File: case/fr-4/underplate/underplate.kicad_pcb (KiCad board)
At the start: 2 copper layers, 152.3 x 104.7 mm, 8 parts

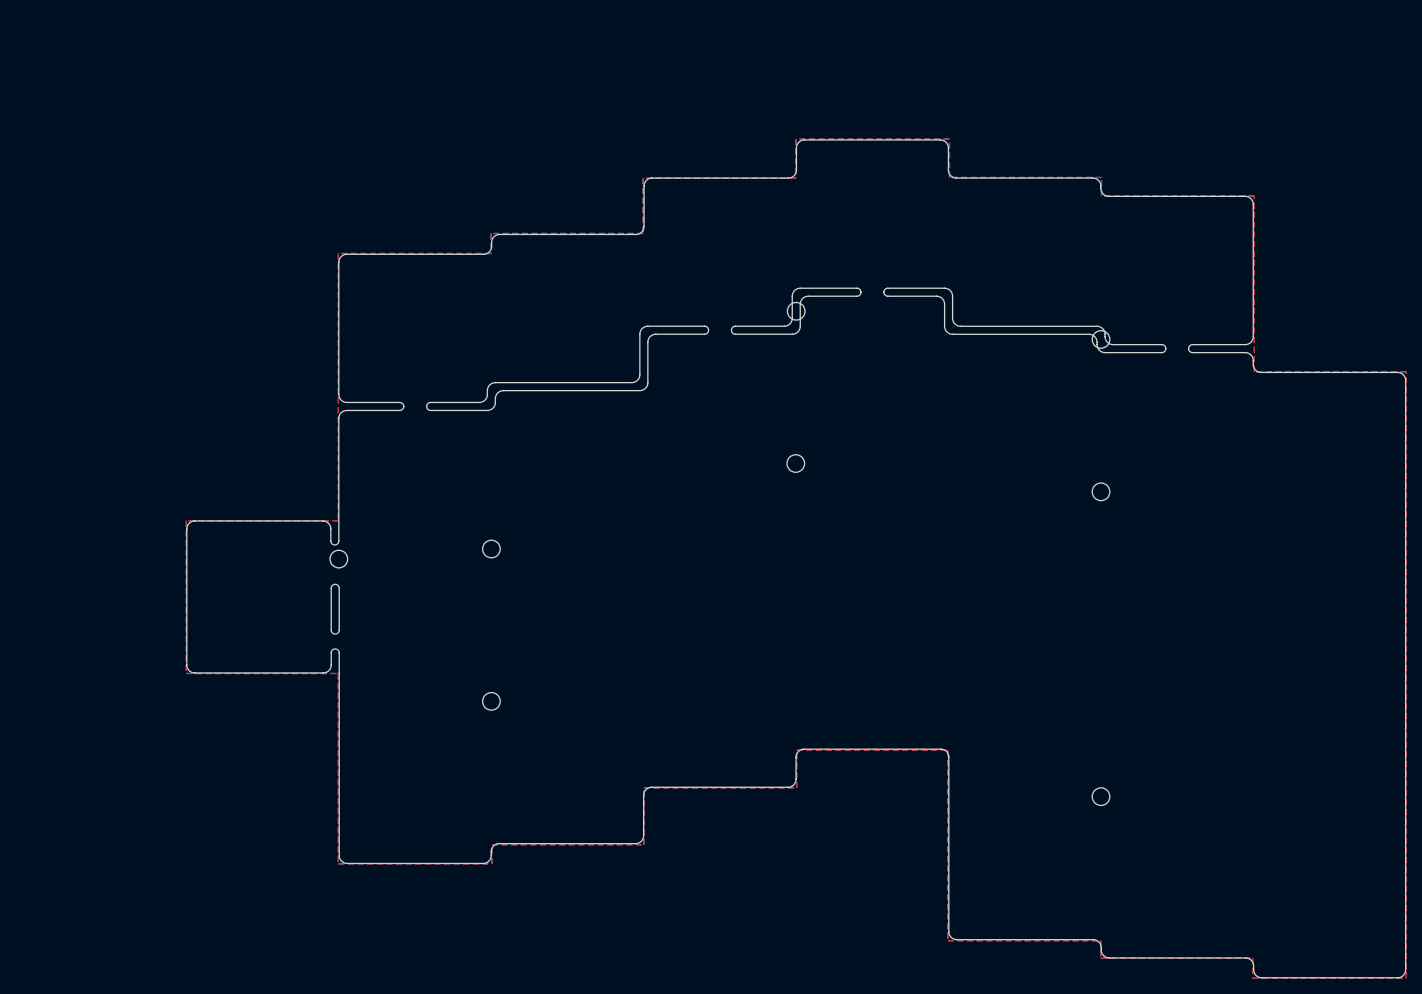
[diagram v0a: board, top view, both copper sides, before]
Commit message: Change screw holes
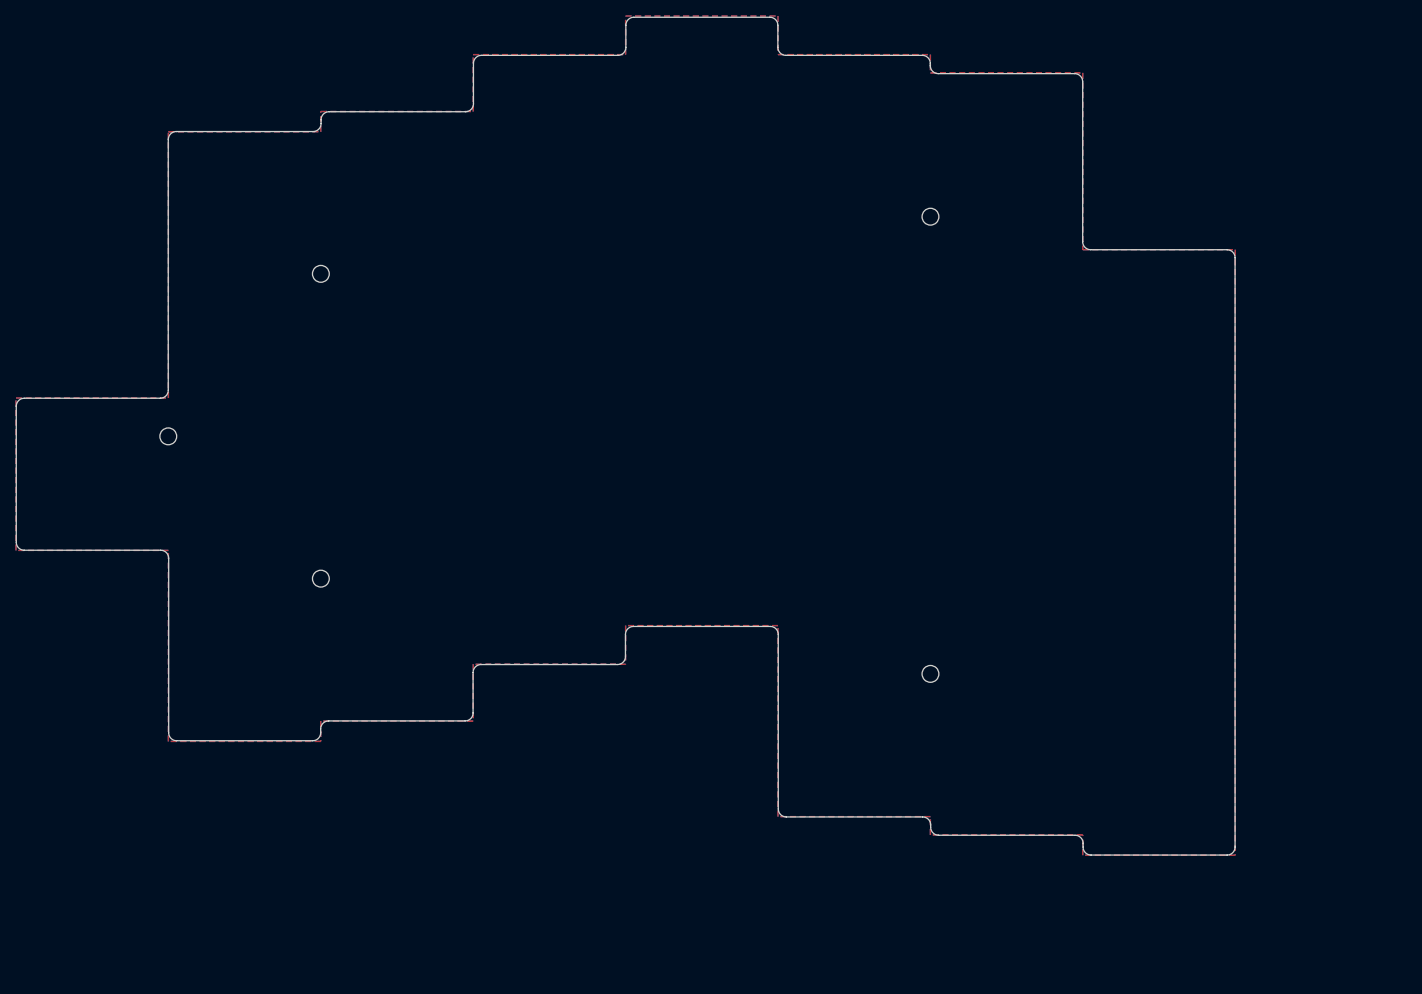
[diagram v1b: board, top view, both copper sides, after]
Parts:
- removed HM1, HM2, HM3, HM4, HM5, HM6, HM7, HM8: CaseHole, Used_Footprints:Hole_Mount_M4
- added REF**: MountingHole_2.1mm, MountingHole:MountingHole_2.1mm, F.Cu at (83.5, 95.2)
- added REF**: MountingHole_2.1mm, MountingHole:MountingHole_2.1mm, F.Cu at (178.8, 124.9)
- added REF**: MountingHole_2.1mm, MountingHole:MountingHole_2.1mm, F.Cu at (178.8, 67.8)
- added REF**: MountingHole_2.1mm, MountingHole:MountingHole_2.1mm, F.Cu at (102.6, 74.9)
- added REF**: MountingHole_2.1mm, MountingHole:MountingHole_2.1mm, F.Cu at (102.6, 113.0)
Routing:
- net (no net): vias 0 -> 1
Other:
- board size 152.3 x 104.7 mm -> 152.4 x 104.7 mm
